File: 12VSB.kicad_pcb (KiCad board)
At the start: 2 copper layers, 24 parts, among them U1 FP6296

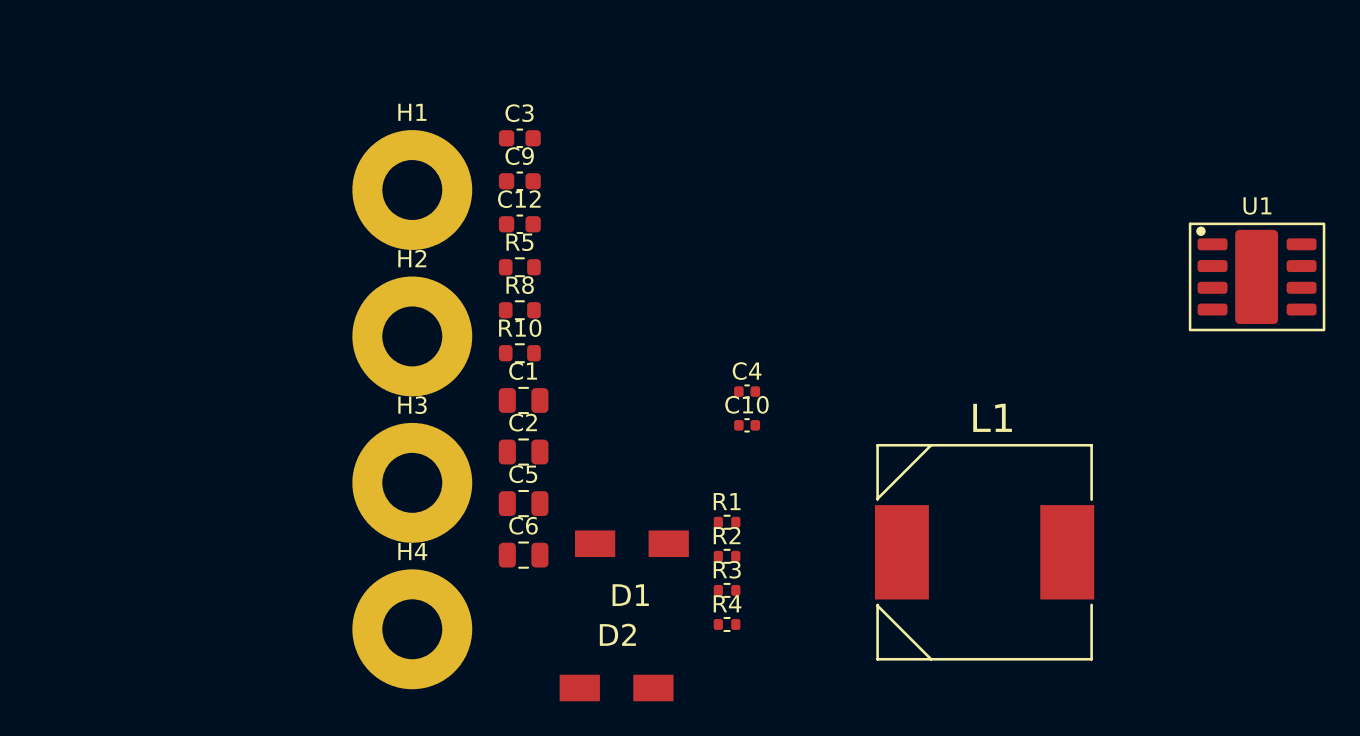
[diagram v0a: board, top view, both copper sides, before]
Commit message: updated pcb layout
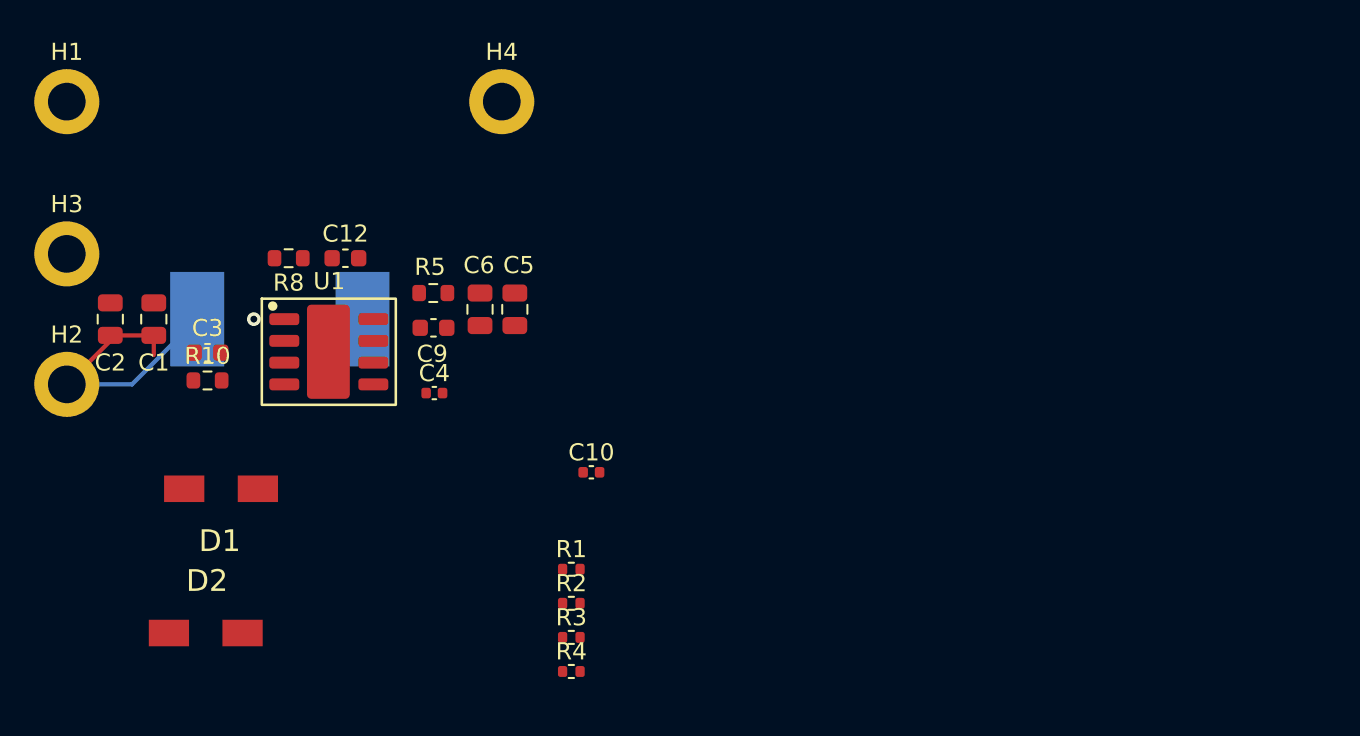
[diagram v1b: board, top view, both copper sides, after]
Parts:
- H1, H2, H3, H4: footprint MountingHole:MountingHole_3.5mm_Pad -> MountingHole:MountingHole_2.2mm_M2_DIN965_Pad
- L1: moved to B.Cu
- moved U1 54.4 mm to (69.9, 65.4)
- moved L1 43.3 mm to (67.1, 63.5)
- moved H4 31.3 mm to (80.0, 50.8)
- moved C2 25.4 mm to (57.1, 63.5), turned to 90 degrees
- moved D1 24.2 mm to (63.6, 73.4)
- moved D2 24.2 mm to (62.7, 81.8)
- moved H3 24.2 mm to (54.6, 59.7)
- moved C3 22.1 mm to (62.8, 65.5)
- moved C1 22.1 mm to (59.7, 63.5), turned to 90 degrees
- moved H1 20.8 mm to (54.6, 50.8)
- moved H2 20.4 mm to (54.6, 67.3)
- moved R10 18.3 mm to (62.8, 67.1)
- moved C4 18.3 mm to (76.1, 67.8)
- moved C6 14.6 mm to (78.7, 62.9), turned to -90 degrees
- moved R8 13.8 mm to (67.6, 59.9), turned to 180 degrees
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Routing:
- net 5VSB: track 0.00 -> 16.8 mm
- net Net-(D1-A): vias 0 -> 1

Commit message: updated pcb layout
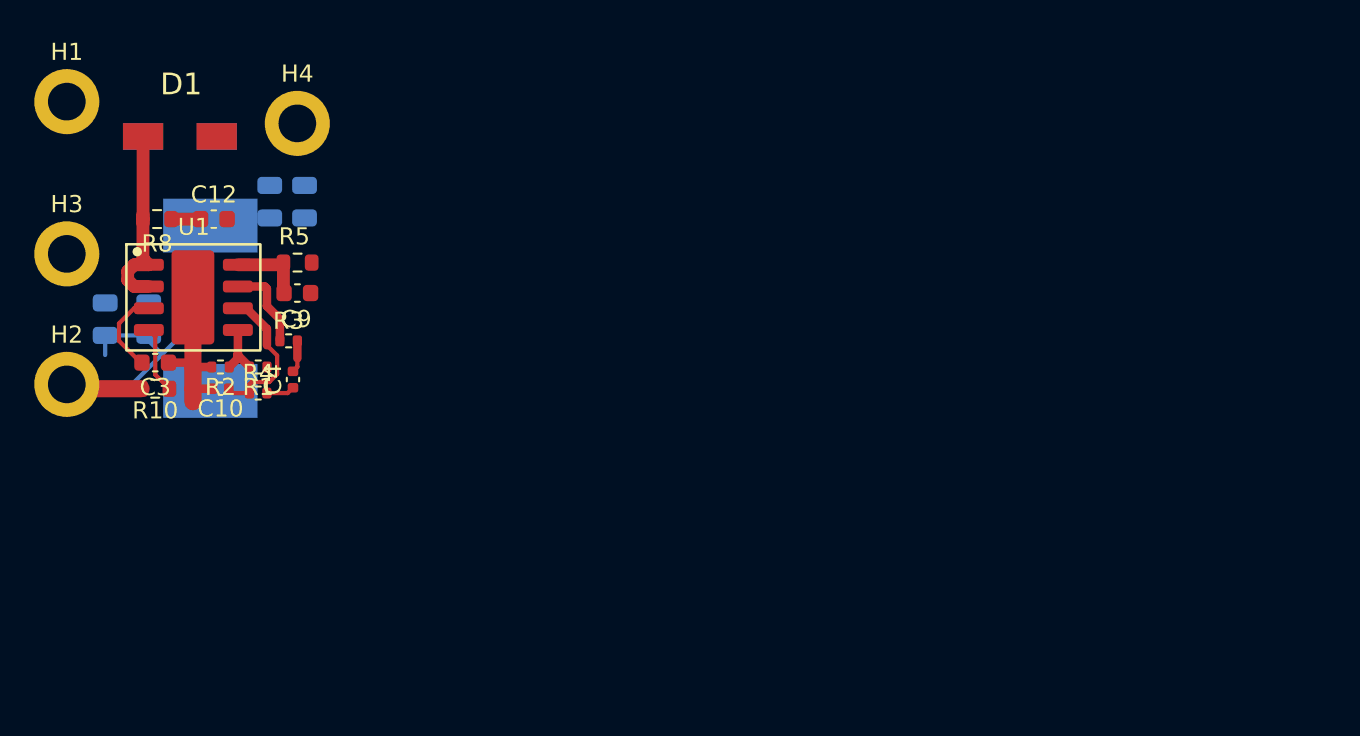
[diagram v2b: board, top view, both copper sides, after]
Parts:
- C1, C2, C5, C6, D2: moved to B.Cu
- moved D2 29.0 mm to (61.2, 52.8)
- moved R2 24.7 mm to (63.6, 66.3), turned to 180 degrees
- moved R4 24.5 mm to (65.8, 67.8)
- moved R3 23.9 mm to (67.6, 64.8)
- moved C10 22.2 mm to (63.6, 67.6), turned to 180 degrees
- moved R1 21.8 mm to (65.8, 66.3), turned to 180 degrees
- moved D1 20.7 mm to (61.2, 52.8), turned to 180 degrees
- moved C5 15.6 mm to (66.5, 56.6)
- moved C6 12.0 mm to (68.5, 56.6)
- moved H4 12.0 mm to (68.1, 52.1)
- moved U1 8.52 mm to (62.0, 62.2)
- moved C4 8.29 mm to (67.8, 67.0), turned to 90 degrees
- moved C9 8.21 mm to (68.1, 62.0)
- moved R5 8.12 mm to (68.1, 60.2)
- moved C12 8.02 mm to (63.2, 57.7)
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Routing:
- net GNDREF: track 0.00 -> 11.7 mm
- net Net-(D1-A): track 0.00 -> 10.9 mm, vias 1 -> 0
- net Net-(U1-COMP): track 0.00 -> 8.77 mm
- net Net-(U1-OC): track 0.00 -> 5.11 mm
- net Net-(U1-VCC): track 0.00 -> 5.00 mm
- net 5VSB: track 16.8 -> 21.6 mm
- net Net-(U1-HVDD): track 0.00 -> 4.50 mm
- net Net-(U1-EN): track 0.00 -> 3.93 mm
- net Net-(U1-FB): track 0.00 -> 3.41 mm
- net Net-(C12-Pad1): track 0.00 -> 1.71 mm
- net Net-(C4-Pad1): track 0.00 -> 1.65 mm
